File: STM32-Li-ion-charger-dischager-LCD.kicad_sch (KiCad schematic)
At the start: 31 parts, among them J4 Conn_01x08, J5 USB_B_Mini, SW4 SW_SPDT, U1 STM32L151C6Ux, Y1 32k, Y2 32k

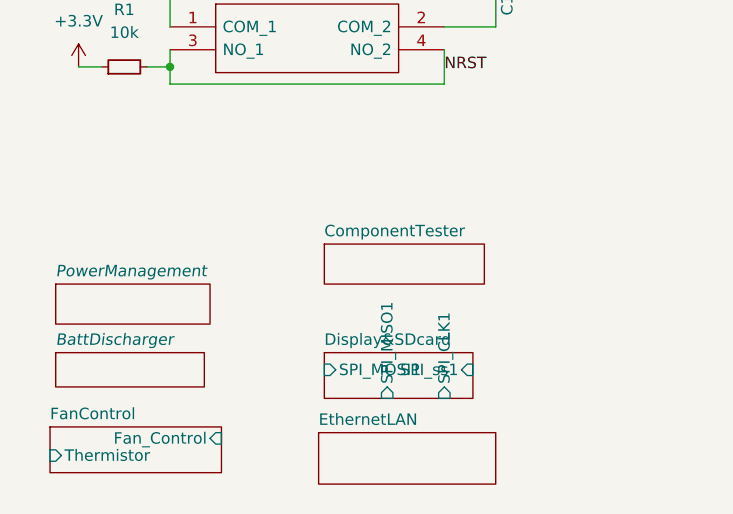
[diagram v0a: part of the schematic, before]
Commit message: j
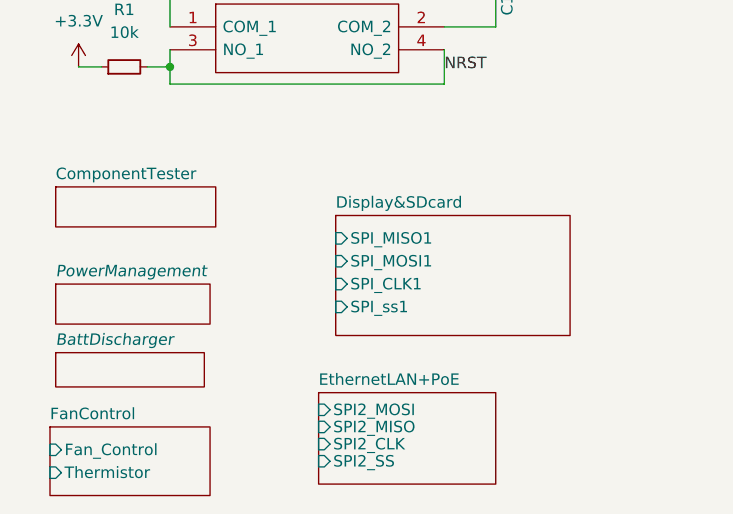
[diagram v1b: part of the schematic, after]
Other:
- sheet EthernetLAN renamed EthernetLAN+PoE
- sheet EthernetLAN+PoE ports: added SPI2_CLK, SPI2_MISO, SPI2_MOSI, SPI2_SS; removed none

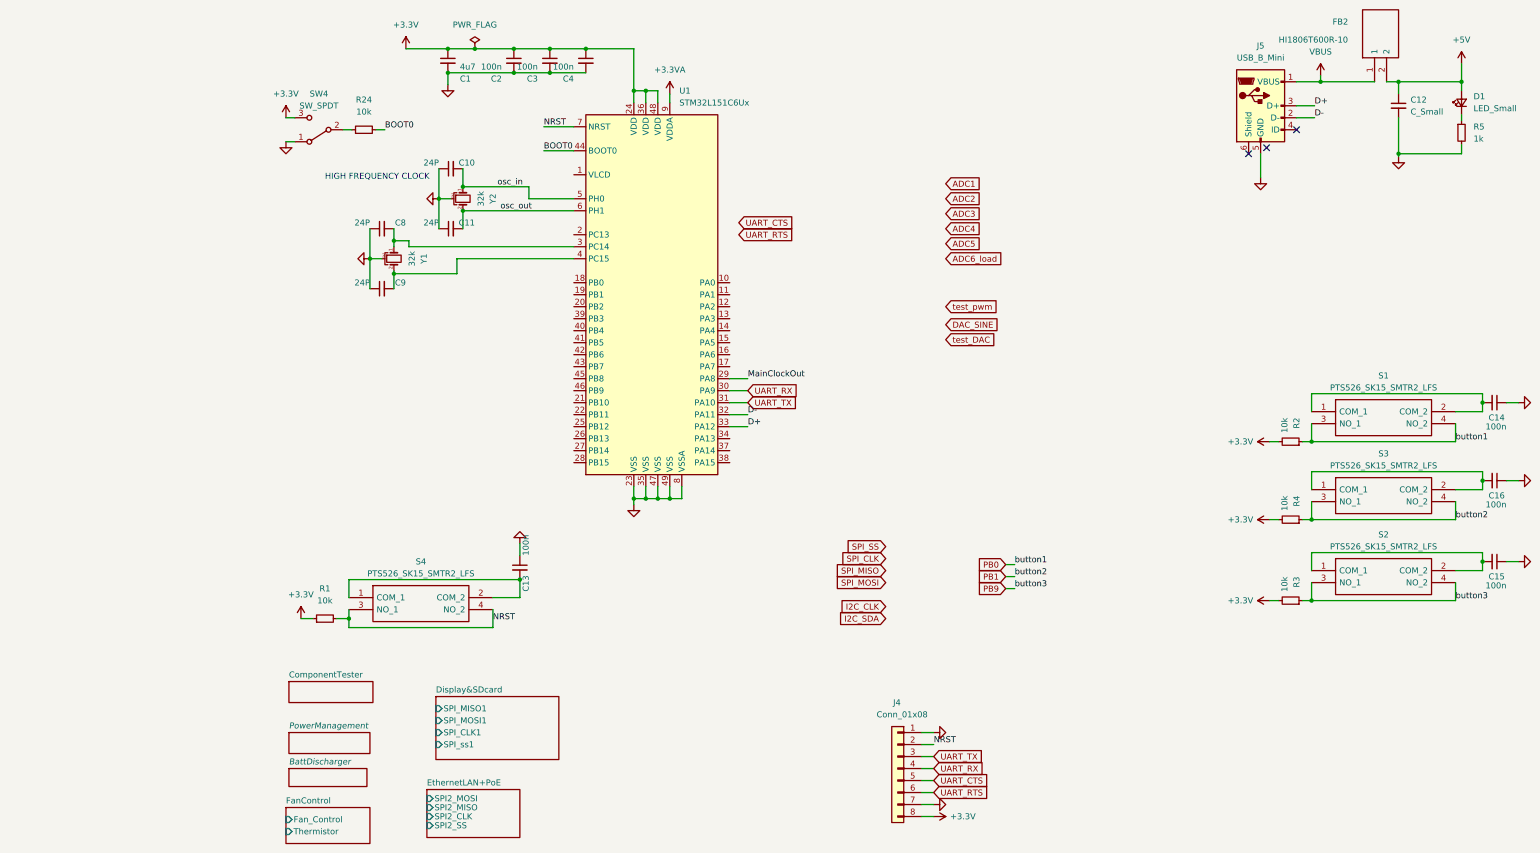
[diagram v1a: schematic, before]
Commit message: more work
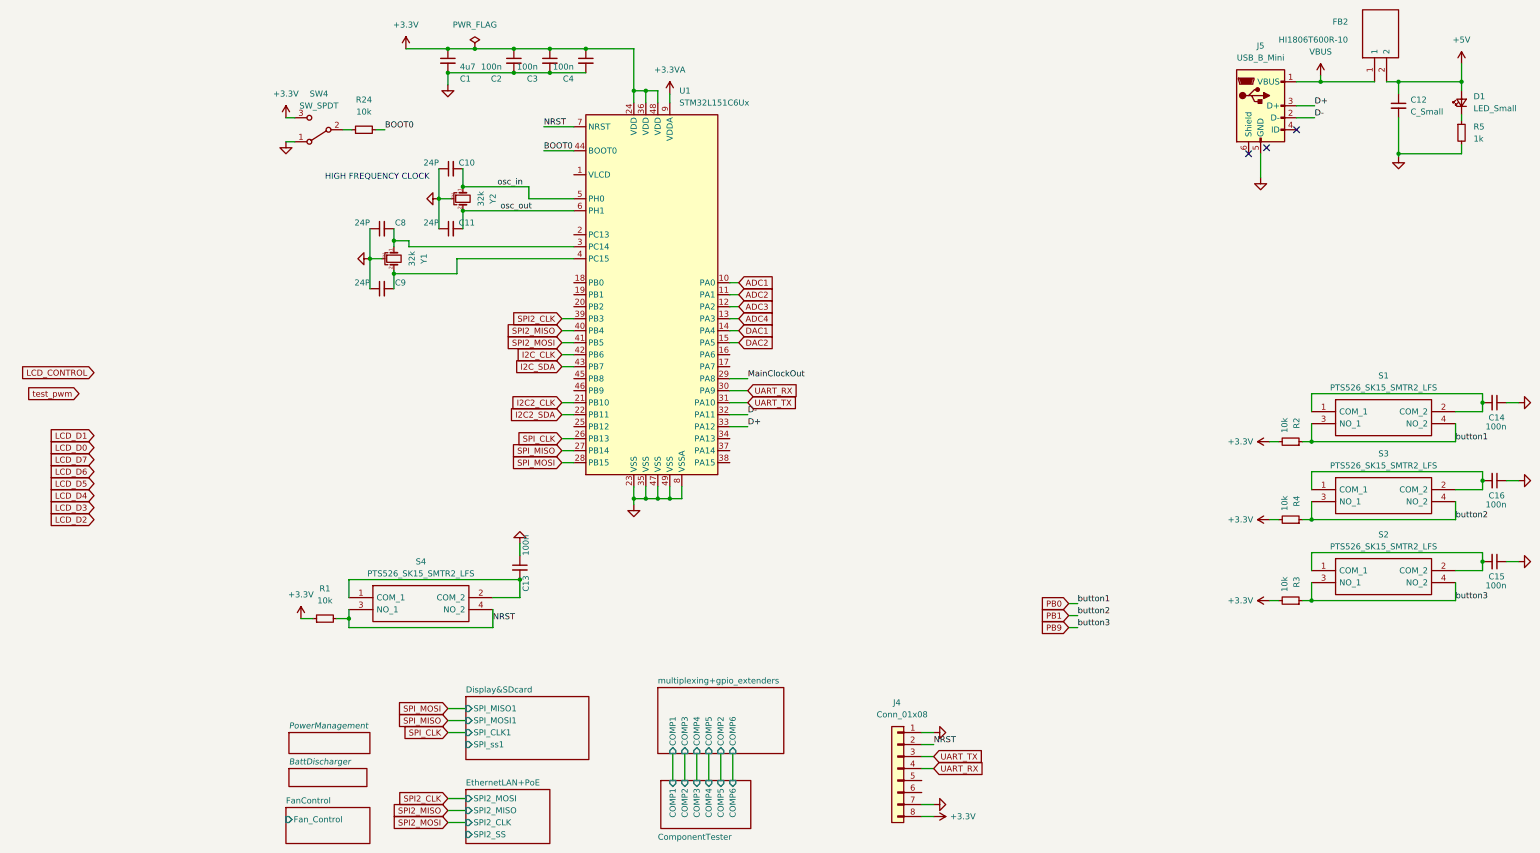
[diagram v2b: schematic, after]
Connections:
- net ADC1: now also U1.10 (PA0)
- net ADC2: now also U1.11 (PA1)
- net ADC3: now also U1.12 (PA2)
- net ADC4: now also U1.13 (PA3)
- net I2C_CLK: now also U1.42 (PB6)
- net I2C_SDA: now also U1.43 (PB7)
- net SPI_CLK: now also U1.26 (PB13)
- net SPI_MISO: now also U1.27 (PB14)
- net SPI_MOSI: now also U1.28 (PB15)
- net DAC1: now reaches U1.14 (PA4)
- net DAC2: now reaches U1.15 (PA5)
- net I2C2_CLK: now reaches U1.21 (PB10)
- net I2C2_SDA: now reaches U1.22 (PB11)
- net SPI2_CLK: now reaches U1.39 (PB3)
- net SPI2_MISO: now reaches U1.40 (PB4)
- net SPI2_MOSI: now reaches U1.41 (PB5)
- net UART_CTS: no longer names the net of J4.5 (Pin_5)
- net UART_RTS: no longer names the net of J4.6 (Pin_6)
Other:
- added sheet multiplexing+gpio_extenders (multiplexing+gpio_extenders.kicad_sch)
- sheet ComponentTester ports: added COMP1, COMP2, COMP3, COMP4, COMP5, COMP6; removed none
- sheet FanControl ports: added none; removed Thermistor

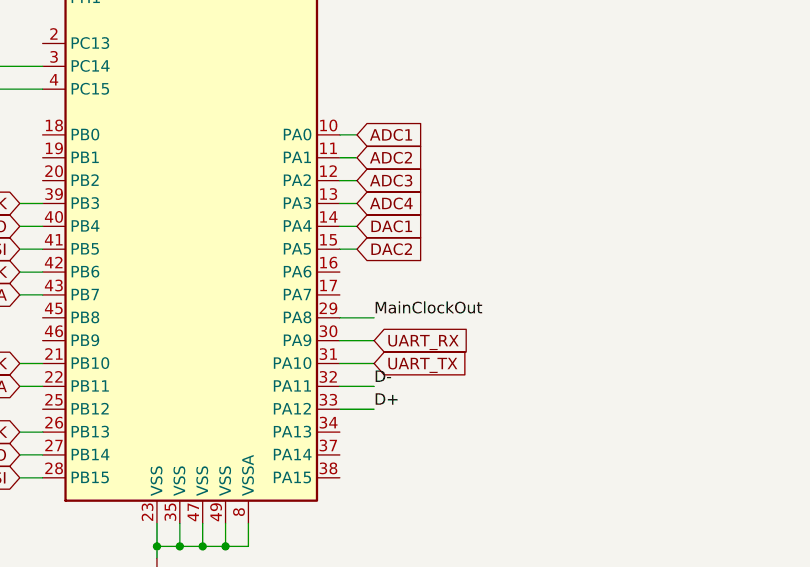
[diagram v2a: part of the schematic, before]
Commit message: h
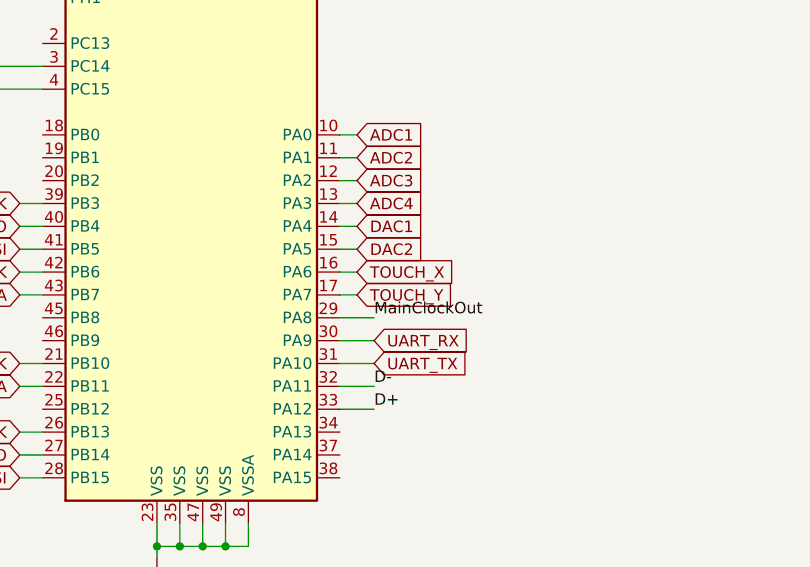
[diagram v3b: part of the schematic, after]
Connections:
- net TOUCH_X: now reaches U1.16 (PA6)
- net TOUCH_Y: now reaches U1.17 (PA7)
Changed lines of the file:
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@@
+    (stroke (width 0) (type default) (color 0 0 0 0))
+  )
+  (wire (pts (xy 111.76 93.345) (xy 113.665 93.345))
     (stroke (width 0) (type default) (color 0 0 0 0))
   )
@@
   )
   (wire (pts (xy 66.04 31.115) (xy 52.07 31.115))
+    (stroke (width 0) (type default) (color 0 0 0 0))
+  )
+  (wire (pts (xy 111.76 90.805) (xy 113.665 90.805))
     (stroke (width 0) (type default) (color 0 0 0 0))
   )
@@
     )
   )
+  (global_label "TOUCH_X" (shape input) (at 113.665 90.805 0) (fields_autoplaced)
+    (effects (font (size 1.27 1.27)) (justify left))
+    (property "Intersheet References" "${INTERSHEET_REFS}" (id 0) (at 124.4843 90.8844 0)
+      (effects (font (size 1.27 1.27)) (justify left) hide)
+    )
+  )
   (global_label "SPI_CLK" (shape input) (at 52.07 170.815 180) (fields_autoplaced)
     (effects (font (size 1.27 1.27)) (justify right))
@@
     (property "Intersheet References" "${INTERSHEET_REFS}" (id 0) (at -32.2883 118.0306 0)
       (effects (font (size 1.27 1.27)) (justify right) hide)
+    )
+  )
+  (global_label "TOUCH_Y" (shape input) (at 113.665 93.345 0) (fields_autoplaced)
+    (effects (font (size 1.27 1.27)) (justify left))
+    (property "Intersheet References" "${INTERSHEET_REFS}" (id 0) (at 124.3633 93.4244 0)
+      (effects (font (size 1.27 1.27)) (justify left) hide)
     )
   )
@@
       (reference "IC4") (unit 1) (value "PEC12R-4230F-S0024") (footprint "PEC12R4230FS0024")
     )
+    (path "/9ca66431-4ae9-450d-a902-4ddfe318c744/1b0dc7d9-bdd8-4cc3-b800-a9d936cb284f"
+      (reference "IC?") (unit 1) (value "XRA1203IG24TR-F") (footprint "SOP65P640X120-24N")
+    )
     (path "/9ba7dc72-30ab-459c-b7f7-117aa274a468/f868776f-0ad2-4ffe-b528-607ce6660028"
       (reference "J1") (unit 1) (value "Conn_01x02") (footprint "Connector_PinHeader_2.54mm:PinHeader_1x02_P2.54mm_Vertical")
@@
       (reference "U11") (unit 1) (value "OPA188xxD") (footprint "Package_SO:SOIC-8_3.9x4.9mm_P1.27mm")
     )
-    (path "/9ca66431-4ae9-450d-a902-4ddfe318c744/4c726e0f-1585-43bc-ab71-e97533286e72"
-      (reference "U12") (unit 1) (value "CD4052B") (footprint "")
-    )
-    (path "/9ca66431-4ae9-450d-a902-4ddfe318c744/a8a0c780-e374-4b11-9834-fa797484e09e"
-      (reference "U13") (unit 1) (value "CD4052B") (footprint "")
+    (path "/9ca66431-4ae9-450d-a902-4ddfe318c744/6a9a2704-c264-456d-91fc-0c962ac61b47"
+      (reference "U?") (unit 1) (value "MC74VHC4052DR2G") (footprint "Package_SO:SOIC-16_3.9x9.9mm_P1.27mm")
+    )
+    (path "/9ca66431-4ae9-450d-a902-4ddfe318c744/71ebeb77-bc54-43d0-bad6-45405931d085"
+      (reference "U?") (unit 1) (value "MC74VHC4052DR2G") (footprint "Package_SO:SOIC-16_3.9x9.9mm_P1.27mm")
     )
     (path "/4849788e-5e45-4118-835e-f9b9ea5fb3c9"
